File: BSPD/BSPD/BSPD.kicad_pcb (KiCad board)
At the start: 2 copper layers, 44 x 36 mm, 47 parts, among them J1 430450613, K1 AZ943-1CH-12DE, U3 74HC1G08GW_125, U4 74HC1G02GW_125, U5 LTC6994CS6-1-TRMPBF, U6 DRDC3105F-7, U7 UA78M05CDCYR, U9 74HC32D_653

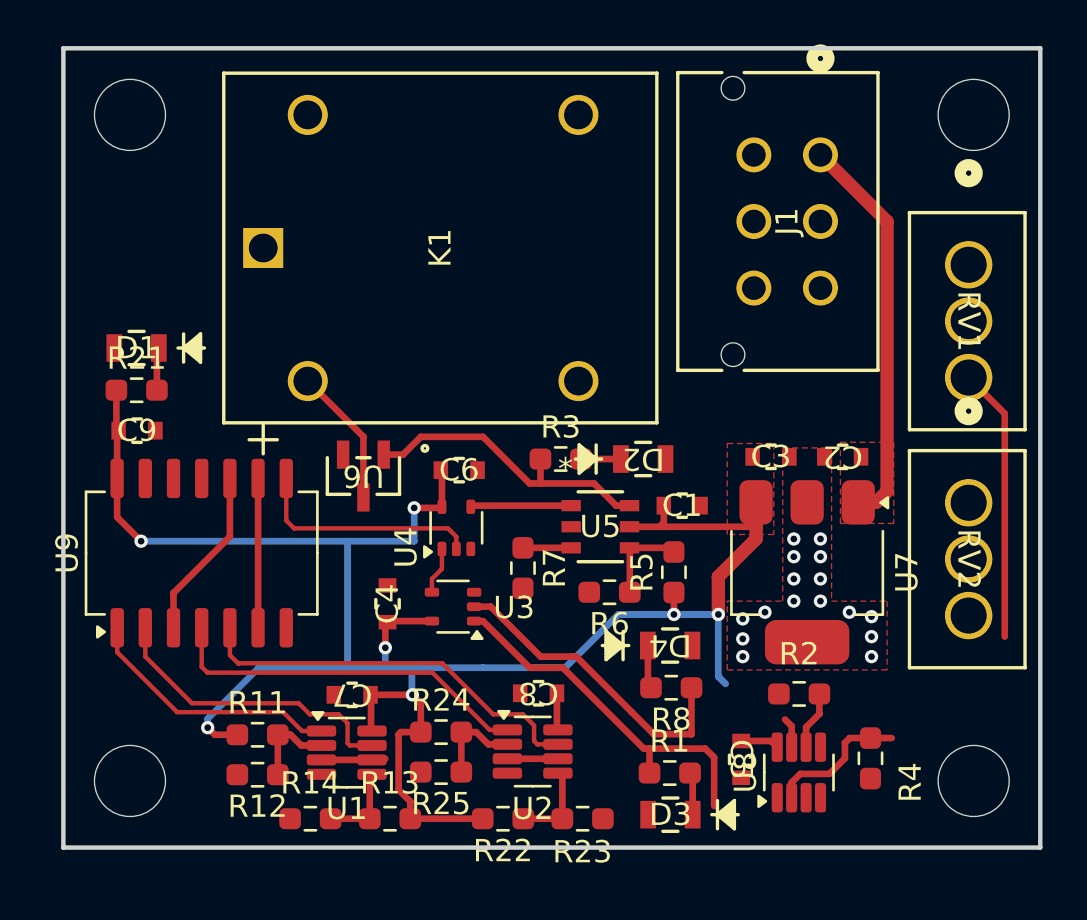
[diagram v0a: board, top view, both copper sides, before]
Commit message: Update
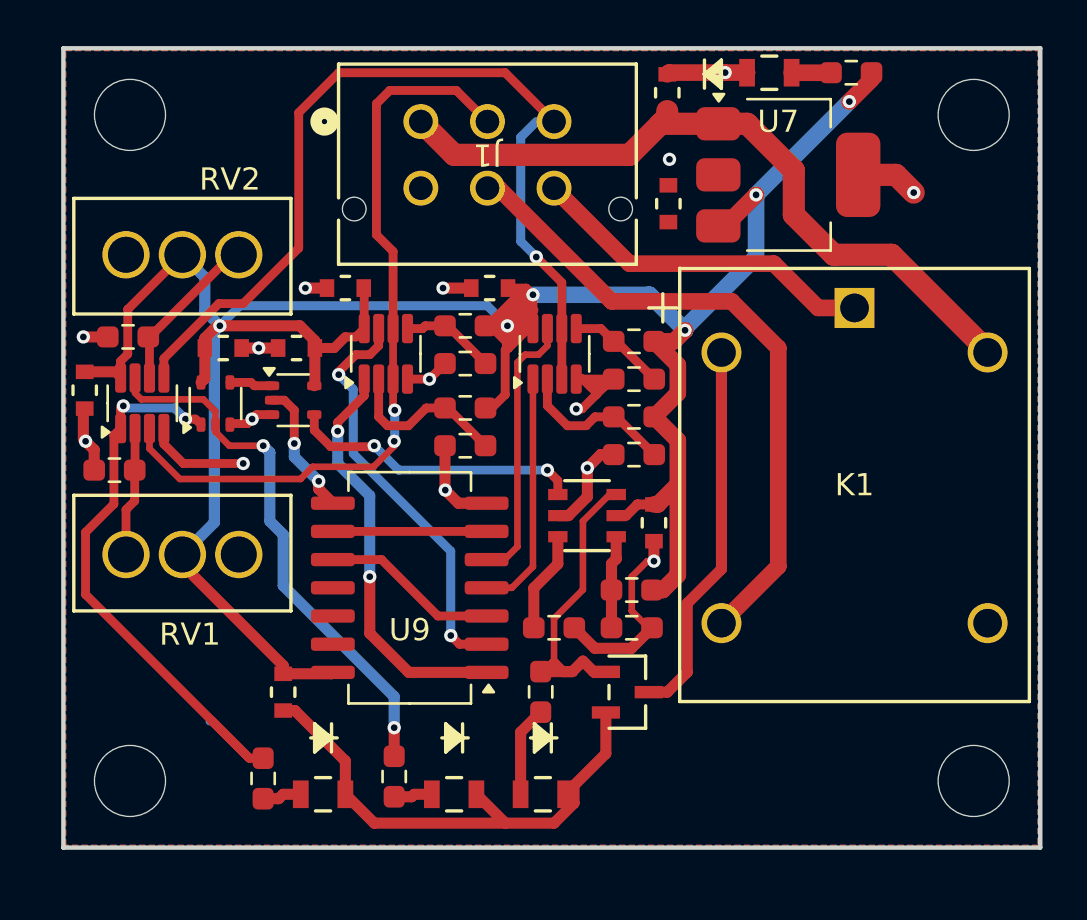
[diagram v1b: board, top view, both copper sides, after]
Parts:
- moved RV2 39.6 mm to (53.8, 68.3), turned to 0 degrees
- moved R4 36.4 mm to (53.3, 78.0), turned to 180 degrees
- moved RV1 35.4 mm to (58.9, 81.8), turned to 180 degrees
- moved R21 35.2 mm to (86.5, 60.1), turned to 180 degrees
- moved R2 34.2 mm to (53.9, 72.0)
- moved U8 33.9 mm to (54.6, 75.0)
- moved C5 33.9 mm to (52.0, 74.4)
- moved D1 31.1 mm to (82.8, 60.1)
- moved K1 26.8 mm to (86.6, 70.7), turned to 0 degrees
- moved R13 22.5 mm to (69.1, 71.5)
- moved R22 22.3 mm to (76.7, 72.2), turned to 180 degrees
- moved R14 21.7 mm to (69.1, 73.2)
- moved R23 19.9 mm to (76.7, 73.9), turned to 180 degrees
- moved C8 18.4 mm to (70.2, 69.8)
- moved C7 18.3 mm to (63.7, 69.8)
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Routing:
- net GND: track 0.00 -> 70.8 mm, vias 16 -> 15
- net Current Sense: track 2.28 -> 41.7 mm, vias 0 -> 1
- net Brake Sense: track 2.90 -> 34.6 mm, vias 0 -> 2
- net /Shutdown Out: track 0.00 -> 29.5 mm
- net +5V: track 95.7 -> 123.7 mm, vias 7 -> 6
- net /Shutdown In: track 0.00 -> 15.8 mm
- net +12V: track 17.9 -> 32.9 mm
- net Net-(U8-INA-): track 18.8 -> 5.84 mm
- net Net-(U6-OUT): track 6.32 -> 17.1 mm
- net /Brake Applied: track 16.6 -> 26.6 mm, vias 0 -> 2
- net /Current Applied: track 15.7 -> 24.4 mm, vias 0 -> 2
- net Net-(U4-Y): track 4.54 -> 13.3 mm, vias 0 -> 2
- net /FaultDetection/Brake Over: track 11.8 -> 18.5 mm, vias 0 -> 2
- net /FaultDetection/Current Over: track 16.8 -> 10.9 mm
- net /FaultDetection/Current Under: track 18.1 -> 12.5 mm
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- removed copper zone on F.Cu, net +12V
- removed copper zone on F.Cu, net +5V
